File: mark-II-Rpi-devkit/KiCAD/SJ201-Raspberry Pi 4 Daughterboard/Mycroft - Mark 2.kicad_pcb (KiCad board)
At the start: 4 copper layers, 72 x 93 mm, 216 parts, among them J1 Barrel_Jack, J10 Debug Connector, J11 I2S, J12 GND, J2 PVDD Jumper, J3 SPKLEFT, J4 SPKRIGHT, J5 PowerTP, J6 Raspberry_Pi_4, J7 USB_B_Micro, J8 MIC, J9 AudioJack3_Ground_Switch, P1 LED, P2 LED, P3 LED, P4 LED, Q3 AO3415A, Q4 FDV301N, SW1 MuteMic, U1 XL4501E1, U10 SPK0838HT4H-1, U11 SPK0838HT4H-1, U12 NCP303LSN09, U13 CM108B, U2 NCP303LSN09, U3 MAX9744, U4 AZ1117CH-3.3, U5 SN74LVC125APWR, U6 FE1.1s, U7 MP2359, U8 XMOS-XVF3510, U9 AT25SF161 16MBIT, X1 SG-210STF 24M, Y2 12MHz

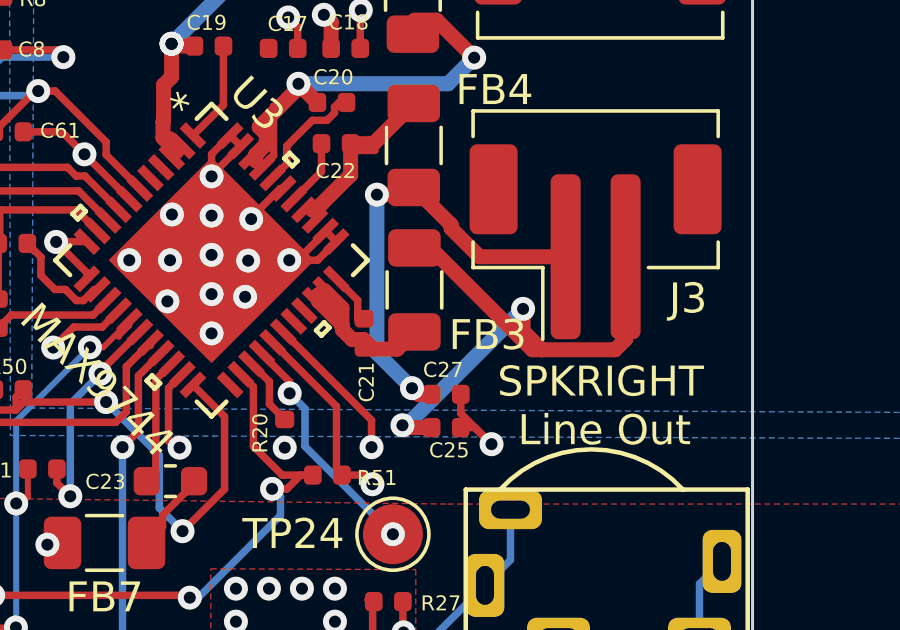
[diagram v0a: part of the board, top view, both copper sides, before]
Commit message: Fix missing items in schematic in Github
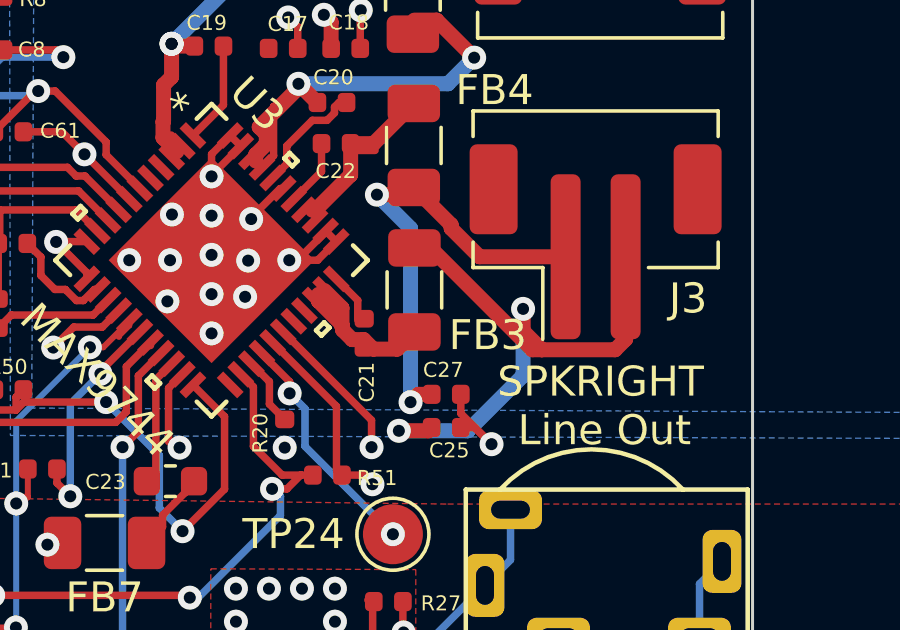
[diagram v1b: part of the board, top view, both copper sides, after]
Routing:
- net Net-(C25-Pad1): track 19.8 -> 21.5 mm
- net Net-(C27-Pad2): track 15.3 -> 15.9 mm
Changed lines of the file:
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@@
     (thickness 1.6)
     (drawings 1914)
-    (tracks 2851)
+    (tracks 2852)
     (zones 0)
     (modules 216)
@@
     (0 F.Cu signal)
     (1 In1.Cu power hide)
-    (2 In2.Cu power)
+    (2 In2.Cu power hide)
     (31 B.Cu signal)
     (32 B.Adhes user hide)
     (33 F.Adhes user hide)
-    (34 B.Paste user)
-    (35 F.Paste user hide)
+    (34 B.Paste user hide)
+    (35 F.Paste user)
     (36 B.SilkS user hide)
     (37 F.SilkS user)
-    (38 B.Mask user)
-    (39 F.Mask user hide)
+    (38 B.Mask user hide)
+    (39 F.Mask user)
     (40 Dwgs.User user hide)
     (41 Cmts.User user hide)
@@
     (46 B.CrtYd user hide)
     (47 F.CrtYd user)
-    (48 B.Fab user)
-    (49 F.Fab user hide)
+    (48 B.Fab user hide)
+    (49 F.Fab user)
   )
   (setup
@@
   (segment (start 64.97657 29.85345) (end 64.3509 29.22778) (width 0.5) (layer F.Cu) (net 70))
   (segment (start 64.3509 29.22778) (end 64.3509 28.49118) (width 0.5) (layer F.Cu) (net 70))
-  (segment (start 64.3509 28.49118) (end 60.47232 32.36976) (width 0.5) (layer B.Cu) (net 70))
-  (via (at 60.33008 32.36976) (size 0.8) (drill 0.4) (layers F.Cu B.Cu) (net 70))
-  (segment (start 60.47232 32.36976) (end 60.33008 32.36976) (width 0.5) (layer B.Cu) (net 70))
-  (segment (start 60.40628 32.44596) (end 60.33008 32.36976) (width 0.5) (layer F.Cu) (net 70))
-  (segment (start 61.30304 32.44596) (end 60.40628 32.44596) (width 0.5) (layer F.Cu) (net 70))
+  (via (at 60.209899 32.554866) (size 0.8) (drill 0.4) (layers F.Cu B.Cu) (net 70))
+  (segment (start 64.3509 30.713957) (end 62.509991 32.554866) (width 0.5) (layer B.Cu) (net 70))
+  (segment (start 61.30304 32.44596) (end 61.194134 32.554866) (width 0.5) (layer F.Cu) (net 70))
+  (segment (start 64.3509 28.49118) (end 64.3509 30.713957) (width 0.5) (layer B.Cu) (net 70))
+  (segment (start 62.509991 32.554866) (end 60.209899 32.554866) (width 0.5) (layer B.Cu) (net 70))
+  (segment (start 61.194134 32.554866) (end 60.209899 32.554866) (width 0.5) (layer F.Cu) (net 70))
   (segment (start 55.694342 15.720158) (end 55.62078 15.79372) (width 0.5) (layer F.Cu) (net 71))
   (segment (start 57.196182 15.720158) (end 55.694342 15.720158) (width 0.5) (layer F.Cu) (net 71))
@@
   (segment (start 62.899724 26.75344) (end 65.76898 26.75344) (width 0.5) (layer F.Cu) (net 72))
   (segment (start 60.70854 24.44288) (end 61.95387 25.68821) (width 0.5) (layer F.Cu) (net 72))
-  (segment (start 59.47918 29.962892) (end 60.648846 31.132558) (width 0.5) (layer B.Cu) (net 72))
-  (segment (start 61.30558 31.33852) (end 60.854808 31.33852) (width 0.5) (layer F.Cu) (net 72))
-  (via (at 60.648846 31.132558) (size 0.8) (drill 0.4) (layers F.Cu B.Cu) (net 72))
-  (segment (start 60.854808 31.33852) (end 60.648846 31.132558) (width 0.5) (layer F.Cu) (net 72))
-  (segment (start 59.47918 24.68372) (end 59.47918 29.962892) (width 0.5) (layer B.Cu) (net 72))
+  (segment (start 61.30558 31.33852) (end 60.86148 31.33852) (width 0.5) (layer F.Cu) (net 72))
+  (via (at 60.6 31.6) (size 0.8) (drill 0.4) (layers F.Cu B.Cu) (net 72))
+  (segment (start 59.47918 24.68372) (end 60.6 25.80454) (width 0.5) (layer B.Cu) (net 72))
+  (segment (start 60.86148 31.33852) (end 60.6 31.6) (width 0.5) (layer F.Cu) (net 72))
+  (segment (start 60.6 25.80454) (end 60.6 31.6) (width 0.5) (layer B.Cu) (net 72))
   (via (at 34.43338 29.85453) (size 0.8) (drill 0.4) (layers F.Cu B.Cu) (net 73))
   (segment (start 34.94038 30.36153) (end 34.43338 29.85453) (width 0.25) (layer B.Cu) (net 73))
